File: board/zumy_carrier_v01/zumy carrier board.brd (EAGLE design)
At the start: 54 x 88.9 mm, 16 parts, among them J1 ODROID_POWER, J2 BATT_POWER, M1 POLOLU_STEP_DOWN, M2 ITG/MPU_MODULE, M3 POLOLU_DRV8833_MODULE, SW1 500SSP1S1M6QEA

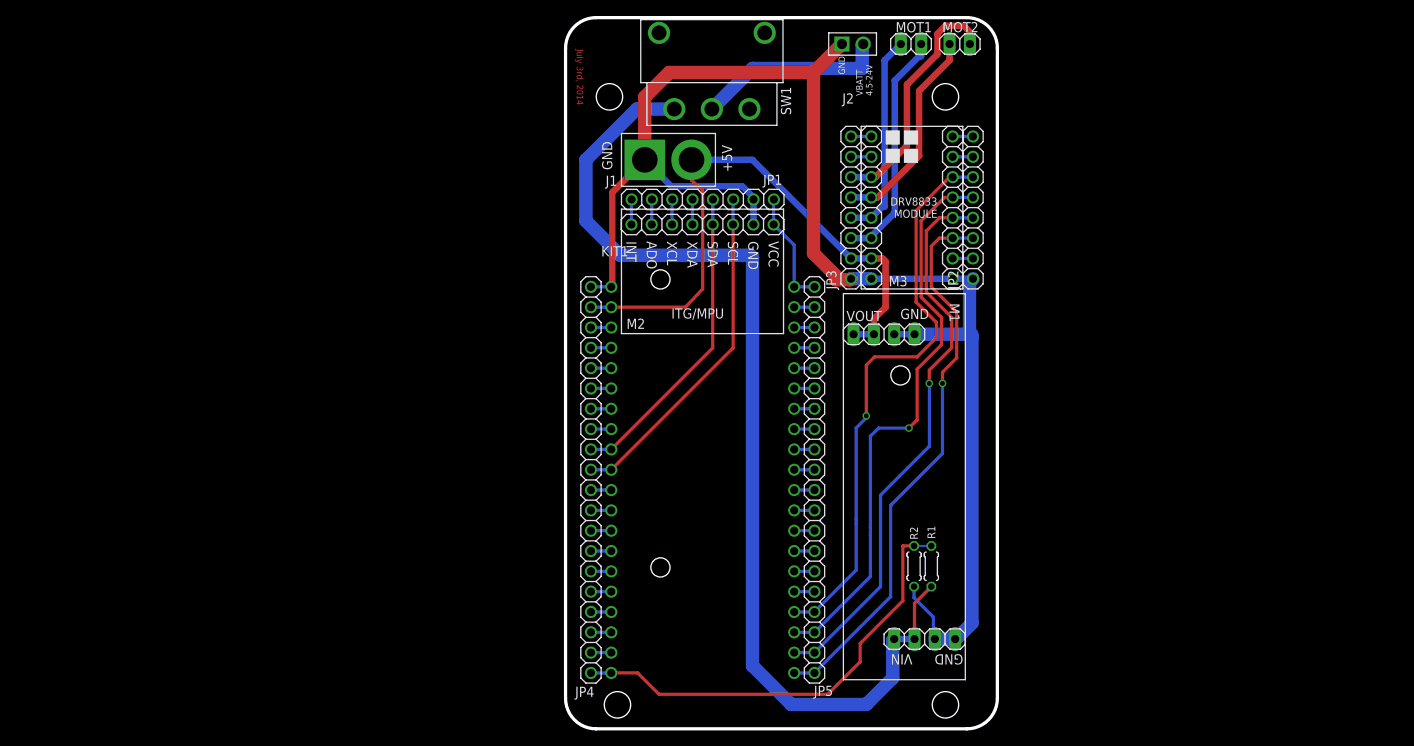
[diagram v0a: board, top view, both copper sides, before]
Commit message: Start of Rev D board. Currently all ripped up.
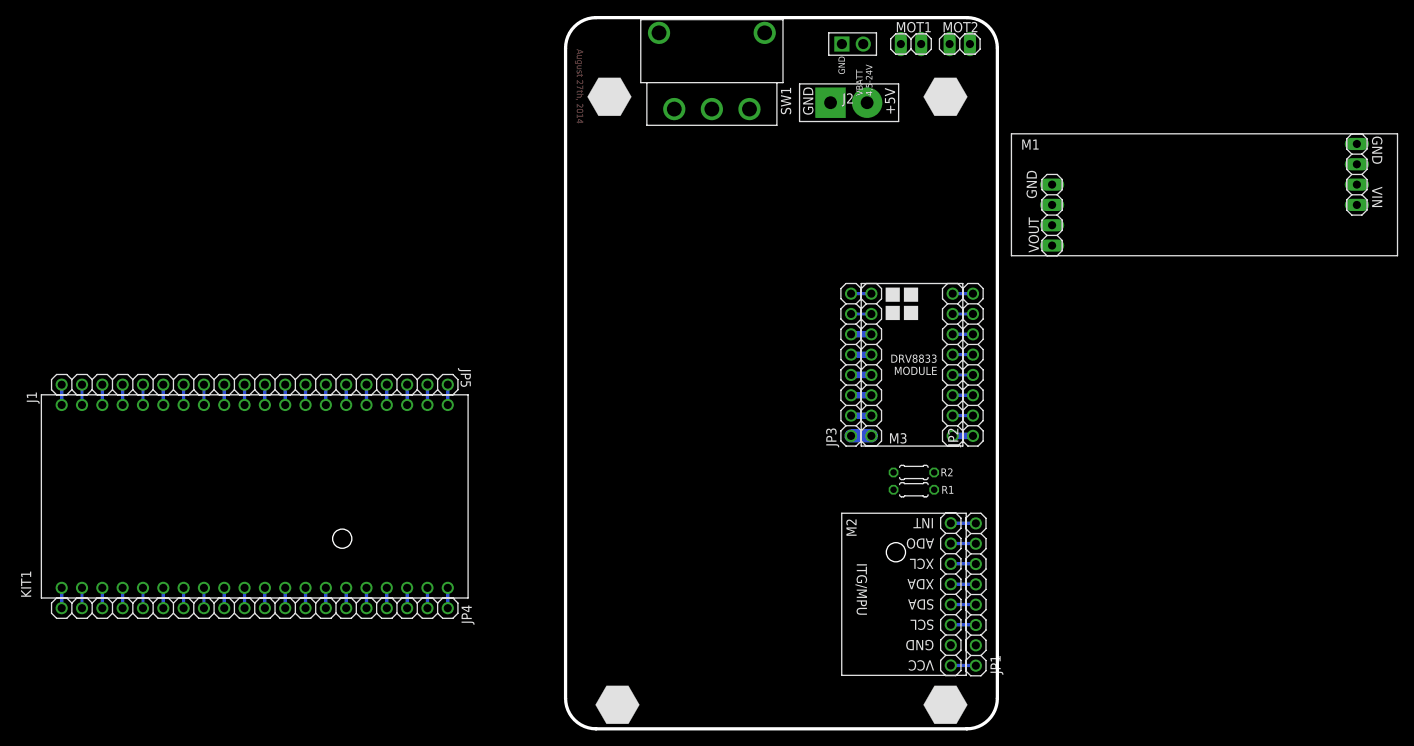
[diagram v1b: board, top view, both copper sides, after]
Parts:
- added U$1, U$2, U$3, U$4: (no value), zumy:STANDOFF_POSITION
- moved JP5 71.0 mm to (-38.9, 43.0), turned to 180 degrees
- moved JP1 60.0 mm to (51.3, 16.8), turned to 270 degrees
- moved KIT1 56.0 mm to (-38.9, 29.1), turned to 90 degrees
- moved M1 52.3 mm to (79.9, 66.8), turned to 0 degrees
- moved M2 45.6 mm to (40.9, 16.8), turned to 270 degrees
- moved JP4 45.0 mm to (-38.9, 15.1), turned to 0 degrees
- moved J1 24.3 mm to (33.1, 78.3)
- moved M3 19.6 mm to (49.7, 55.7)
- moved JP2 19.6 mm to (50.9, 45.5)
- moved JP3 19.6 mm to (35.7, 45.5)
- moved R2 11.7 mm to (43.5, 32.0), turned to 0 degrees
- moved R1 9.81 mm to (43.5, 29.9), turned to 180 degrees
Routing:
- net GND: track 185.3 -> 8.44 mm
- net SW_VBATT: track 130.9 -> 0.00 mm
- net +5V: track 73.5 -> 5.08 mm
- net AIN1: track 72.0 -> 5.08 mm, vias 1 -> 0
- net AIN2: track 71.5 -> 5.08 mm, vias 1 -> 0
- net BIN2: track 70.2 -> 5.08 mm, vias 1 -> 0
- net BIN1: track 70.2 -> 5.08 mm, vias 1 -> 0
- net V_BATT_SENSE: track 56.7 -> 2.54 mm
- net MPU_SCL: track 42.8 -> 5.87 mm
- net MPU_SDA: track 39.2 -> 5.87 mm
- net N$62: track 30.5 -> 2.54 mm
- net N$59: track 29.5 -> 2.54 mm
- net VBATT: track 24.0 -> 0.00 mm
- net N$61: track 26.2 -> 2.54 mm
- net N$60: track 25.9 -> 2.54 mm
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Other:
- board text added: "August 27th, 2014"
- board text added: "Rev D"
- board text removed: "July 3rd, 2014"
- board text removed: "Rev C"
